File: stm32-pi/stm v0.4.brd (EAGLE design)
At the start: 128.9 x 105.8 mm, 144 parts, among them Q1 MMBT3906, Q2 MMBT3904, Q3 MMBT3904, Y1 32.768kHz

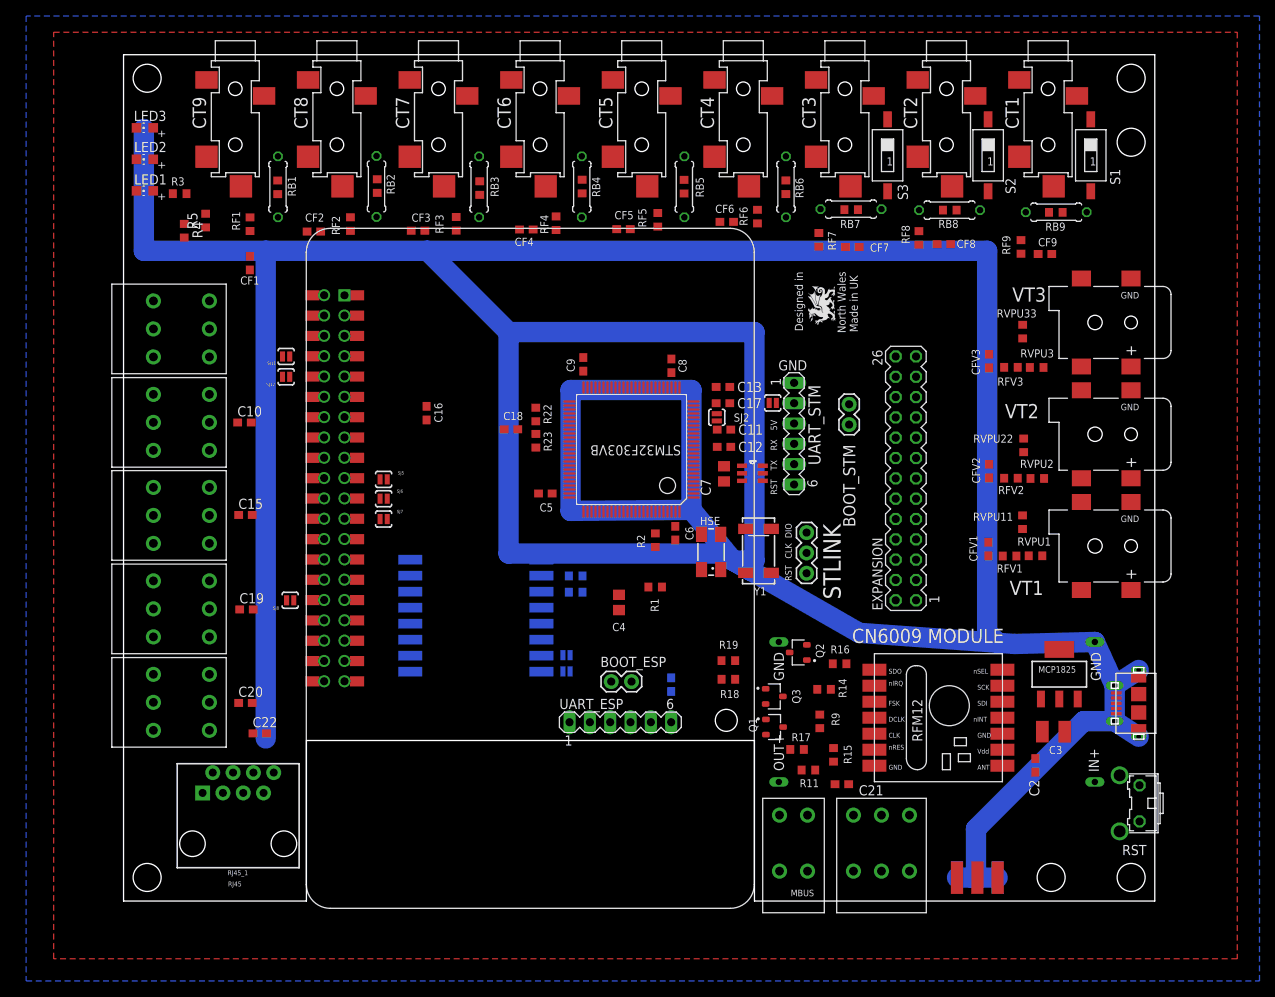
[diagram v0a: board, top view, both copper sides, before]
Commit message: update v0.4
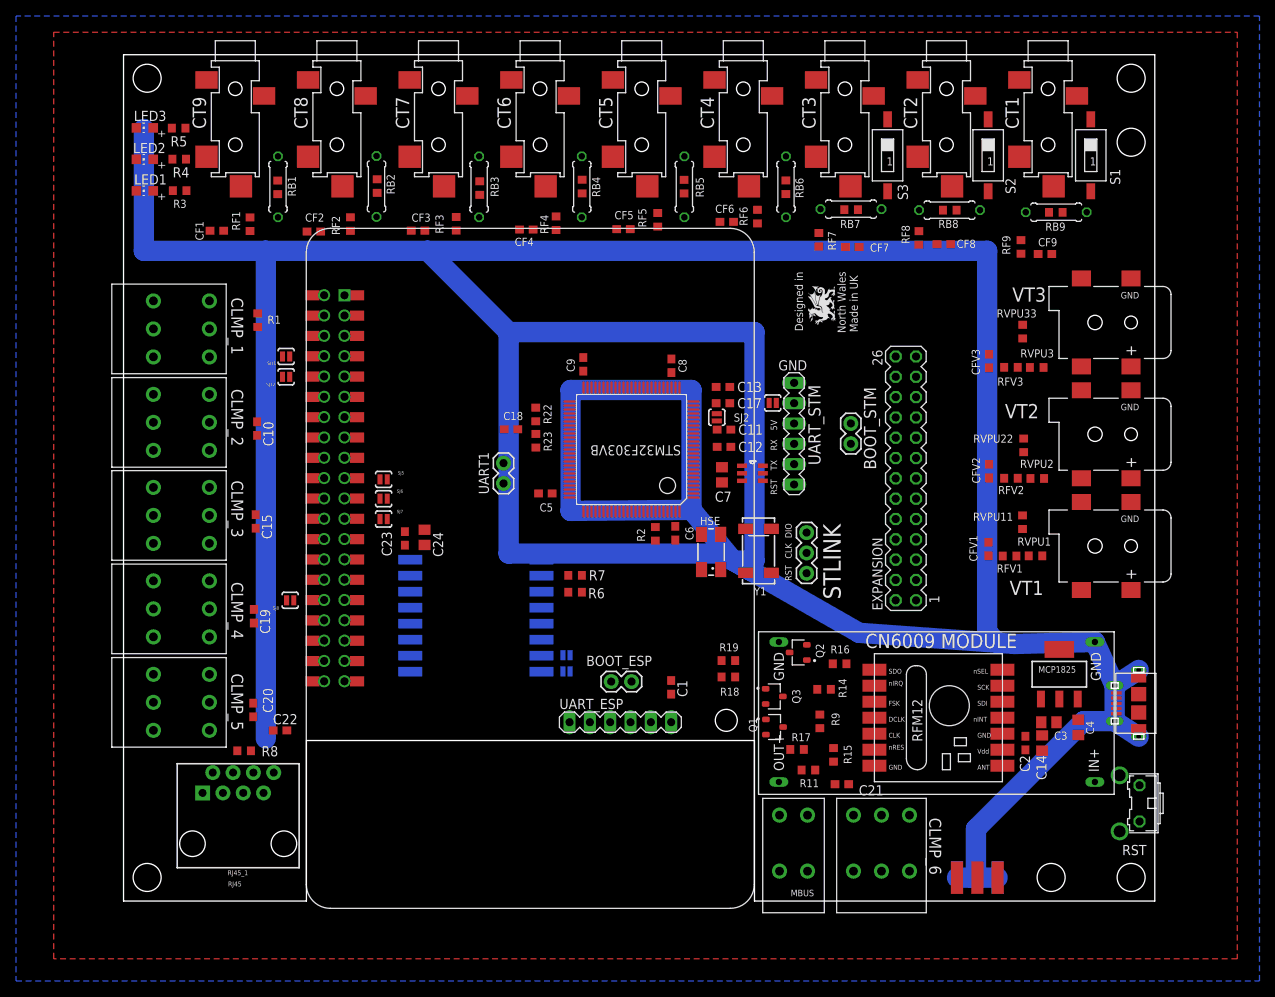
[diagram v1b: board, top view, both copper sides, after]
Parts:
- removed C16: 100nF, resistor:C0603
- added C14: 1uF, rcl:C0805
- added C23: 100nF, resistor:C0603
- added C24: 47uF, rcl:C0805
- added R8: 4.7k, resistor:R0603
- added UART1: (no value), SparkFun:1X02
- C3: device rcl:C1210 -> rcl:C0805
- UART_STM: device con-lstb:MA06-1 -> con-lstb-db:MA06-1
- moved R1 59.8 mm to (16.8, 72.6), turned to 90 degrees
- moved C4 59.5 mm to (119.3, 21.7)
- moved R5 12.0 mm to (6.89, 96.6), turned to 0 degrees
- moved R4 8.97 mm to (6.96, 92.7), turned to 0 degrees
- moved CF1 5.77 mm to (11.7, 83.8), turned to 0 degrees
- moved BOOT_STM 4.94 mm to (90.9, 57.2), turned to 90 degrees
- moved C2 3.05 mm to (112.7, 19.7), turned to 90 degrees
- moved C22 2.57 mm to (19.6, 21.3)
- moved C10 1.76 mm to (16.7, 59.1), turned to 270 degrees
- moved C15 1.52 mm to (16.5, 47.4), turned to 270 degrees
- moved C20 1.32 mm to (16.2, 23.9), turned to 270 degrees
- moved C3 1.32 mm to (115.7, 22.3)
- moved C19 1.25 mm to (16.3, 35.6), turned to 270 degrees
- moved R2 0.79 mm to (66.5, 45.9)
- moved R3 0.38 mm to (7.02, 88.8)
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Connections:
- removed net PULSE: C16.2
- new net UART1_RX: STM32F303VB.69, UART1.1
- new net UART1_TX: STM32F303VB.68, UART1.2
- net +3V3: now also C14.1, C23.1, C24.1, R8.2
- net DS18B20_1: now also 3POLE_1.P$3, 3POLE_1.P$4, STM32F303VB.63; no longer RJ45_1.4
- net DS18B20_2: now also R8.1, RJ45_1.4; no longer 3POLE_1.P$3, 3POLE_1.P$4
- net GND: now also C14.2, C23.2, C24.2; no longer C16.1
- net PULSE2: now also STM32F303VB.67
- net PUSHIN_1: now also STM32F303VB.95
- net PUSHIN_2: now also STM32F303VB.64
- net PUSHIN_3: now also STM32F303VB.65
- net PUSHIN_4: now also STM32F303VB.66
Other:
- board text added: "CLMP_1"
- board text added: "CLMP_2"
- board text added: "CLMP_3"
- board text added: "CLMP_4"
- board text added: "CLMP_5"
- board text added: "CLMP_6"

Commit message: v0.4 update
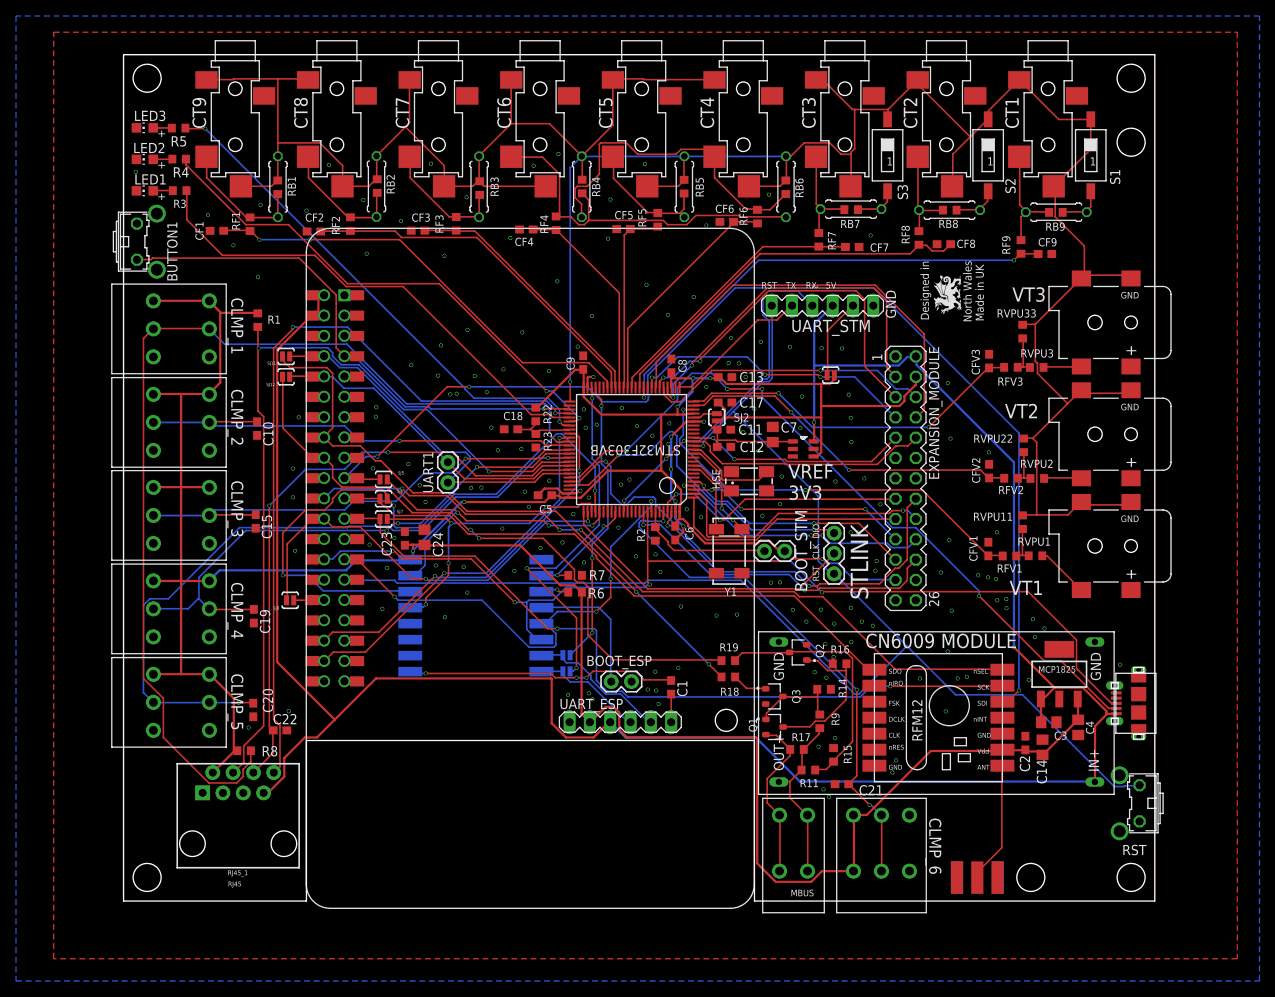
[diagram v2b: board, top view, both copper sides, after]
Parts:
- removed EXPANSION: (no value), con-lstb:MA13-2
- removed U$8: MCP1501T-33E, MCP1501T-33E:SOT95P280X145-6N
- added BUTTON1: (no value), switch-omron:B3F-31XX
- added EXPANSION_MODULE: (no value), con-lstb:MA13-2
- added VREF_3V3: MCP1501T-33E, MCP1501T-33E:SOT95P280X145-6N
- moved BOOT_STM 17.2 mm to (80.1, 43.7), turned to 0 degrees
- moved UART_STM 16.4 mm to (87.4, 74.4), turned to 180 degrees
- moved HSE 10.0 mm to (78.2, 52.5), turned to 0 degrees
- moved C7 8.11 mm to (81.2, 58.3), turned to 90 degrees
- moved SJ1 8.04 mm to (88.4, 65.7), turned to 0 degrees
- moved UART1 6.95 mm to (40.5, 52.3)
- moved Y1 3.67 mm to (75.7, 43.7)
- moved STLINK 3.44 mm to (88.8, 46.0)
- moved C13 1.25 mm to (75.2, 65.5)
- moved C14 0.53 mm to (114.9, 19.2)
- moved C17 0.28 mm to (75.2, 62.3)
- moved C5 0.23 mm to (52.7, 50.7)
- moved C9 0.22 mm to (57.5, 67.3)
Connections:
- removed net DS18B20_1: 3POLE_1.P$3, 3POLE_1.P$4, R1.1, STM32F303VB.63
- removed net N$14: EXPANSION.5
- removed net N$15: EXPANSION.7
- removed net N$17: EXPANSION.9
- removed net N$18: EXPANSION.11
- removed net N$19: EXPANSION.13
- removed net N$20: EXPANSION.15
- removed net N$21: EXPANSION.17
- removed net N$23: EXPANSION.19
- removed net N$25: EXPANSION.21
- removed net N$9: EXPANSION.1
- removed net PULSE1: C22.1, RJ45_1.6
- new net BUTTON1: BUTTON1.2, PCB2.P$47, PCB2.P$7, STM32F303VB.53
- new net DS18B20_RJ45: R1.1, RJ45_1.4, STM32F303VB.66
- new net I010_EX: EXPANSION_MODULE.24
- new net I011_EX: EXPANSION_MODULE.25
- new net IO11_EX: STM32F303VB.95
- new net IO1_EX: EXPANSION_MODULE.15, STM32F303VB.97
- new net IO2_EX: EXPANSION_MODULE.16, STM32F303VB.98
- new net IO3_EX: EXPANSION_MODULE.17, STM32F303VB.1
- new net IO4_EX: EXPANSION_MODULE.18, STM32F303VB.2
- new net IO5_EX: EXPANSION_MODULE.19, STM32F303VB.3
- new net IO6_EX: EXPANSION_MODULE.20, STM32F303VB.4
- new net IO7_EX: EXPANSION_MODULE.21, STM32F303VB.5
- new net IO8_EX: EXPANSION_MODULE.22, STM32F303VB.91
- new net PULSE1_RJ45: C22.1, RJ45_1.6, STM32F303VB.67
- new net RPI_GPIO16: PCB2.P$36, PCB2.P$76, STM32F303VB.59
- new net RPI_GPIO20: PCB2.P$38, PCB2.P$78, STM32F303VB.60
- new net SCK: ESP12.GPIO5, EXPANSION_MODULE.23, PCB2.P$28, PCB2.P$68, STM32F303VB.92
- new net SDA: ESP12.GPIO4, PCB2.P$27, PCB2.P$67, STM32F303VB.93
- new net VT1_EX: EXPANSION_MODULE.11
- new net VT2_EX: EXPANSION_MODULE.12
- new net VT3_EX: EXPANSION_MODULE.13
- net +3V3: now also EXPANSION_MODULE.4, VREF_3V3.4; no longer U$8.4
- net +3V3_ADC: now also VREF_3V3.1; no longer U$8.1
- net +5V: now also EXPANSION_MODULE.2, VREF_3V3.6; no longer U$8.6
- net CT1_EX: now also EXPANSION_MODULE.3
- net CT2_EX: now also EXPANSION_MODULE.6
- net CT3_EX: now also EXPANSION_MODULE.5
- net CT4_EX: now also EXPANSION_MODULE.8
- net CT5_EX: now also EXPANSION_MODULE.7
- net CT6_EX: now also EXPANSION_MODULE.10
- net CT7_EX: now also EXPANSION_MODULE.9
- net DS18B20_2: now also 3POLE_1.P$3, 3POLE_1.P$4, STM32F303VB.61; no longer RJ45_1.4
- net GND: now also BUTTON1.1, EXPANSION_MODULE.1, EXPANSION_MODULE.14, EXPANSION_MODULE.26, VREF_3V3.2, VREF_3V3.3, VREF_3V3.5; no longer U$8.2, U$8.3, U$8.5
- net N$13: now also PCB2.P$26, PCB2.P$66; no longer EXPANSION.3
- net NRST: now also PCB2.P$29, PCB2.P$69
- net PULSE2: now also STM32F303VB.65; no longer STM32F303VB.67
- net PUSHIN_1: now also STM32F303VB.96; no longer STM32F303VB.95
- net PUSHIN_2: now also STM32F303VB.62; no longer STM32F303VB.64
- net PUSHIN_3: now also STM32F303VB.63; no longer STM32F303VB.65
- net PUSHIN_4: now also STM32F303VB.64; no longer STM32F303VB.66
- net SPI3_CS: now also PCB2.P$24, PCB2.P$64
- net UART1_RX: now also PCB2.P$48, PCB2.P$8, SJ11.1
- net UART1_TX: now also PCB2.P$10, PCB2.P$50, SJ12.1
- net USART3_RX: no longer PCB2.P$48, PCB2.P$8, SJ11.1
- net USART3_TX: no longer PCB2.P$10, PCB2.P$50, SJ12.1
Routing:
- net GND: track 533.8 -> 29.1 mm, vias 0 -> 180
- net +3V3: track 0.00 -> 430.2 mm, vias 0 -> 5
- net BIAS: track 0.00 -> 374.6 mm, vias 0 -> 1
- net +5V: track 0.00 -> 286.9 mm, vias 0 -> 2
- net NRST: track 0.00 -> 178.4 mm, vias 0 -> 1
- net MOSI: track 0.00 -> 144.5 mm, vias 0 -> 3
- net DS18B20_2: track 0.00 -> 128.8 mm, vias 0 -> 1
- net DS18B20_RJ45: track 0.00 -> 103.8 mm, vias 0 -> 2
- net SPI_CLK: track 0.00 -> 96.8 mm, vias 0 -> 2
- net ADC_RJ45IN: track 0.00 -> 96.7 mm, vias 0 -> 2
- net CS_RFM69: track 0.00 -> 96.2 mm, vias 0 -> 3
- net SCK: track 0.00 -> 93.4 mm, vias 0 -> 4
- net D-: track 0.00 -> 93.0 mm, vias 0 -> 4
- net D+: track 0.00 -> 87.3 mm, vias 0 -> 2
- net PULSE2: track 0.00 -> 86.6 mm, vias 0 -> 2
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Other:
- board text added: "VREF 3V3"

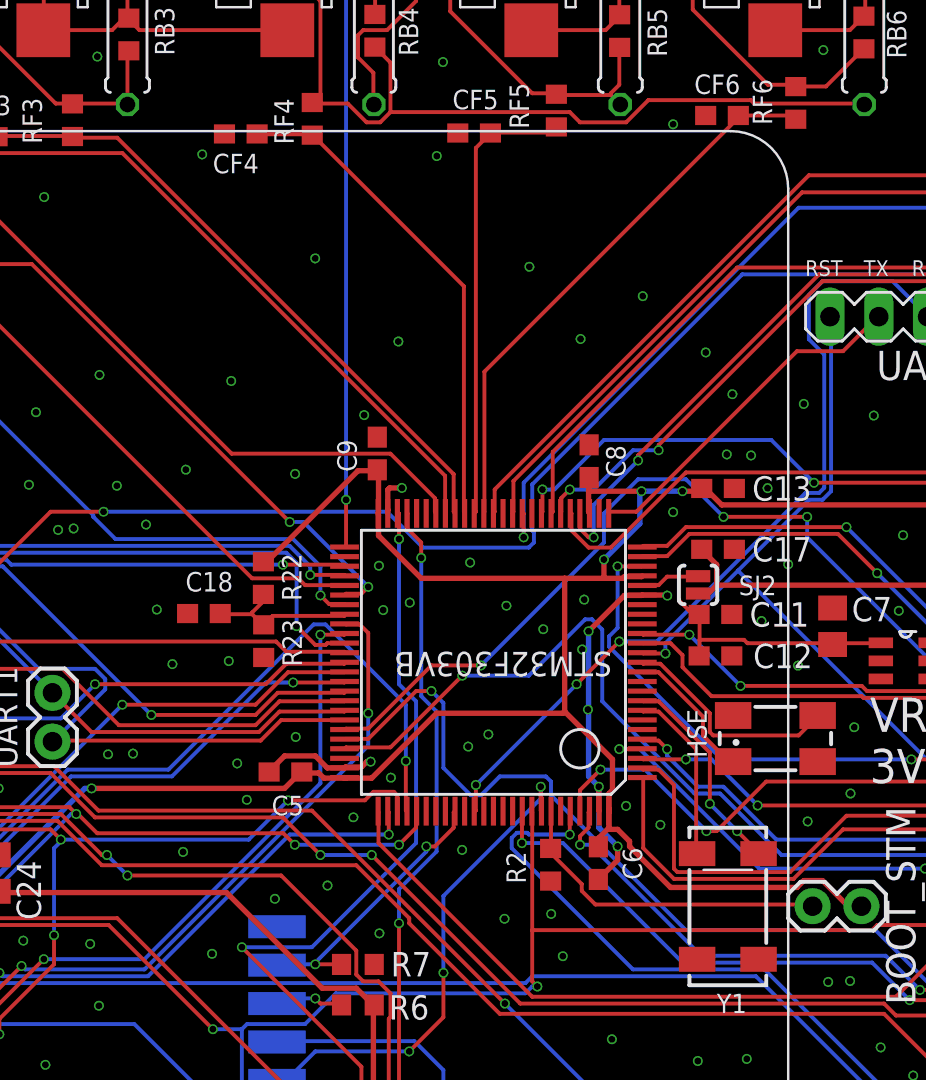
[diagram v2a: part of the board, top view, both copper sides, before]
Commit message: v0.4 update
checked
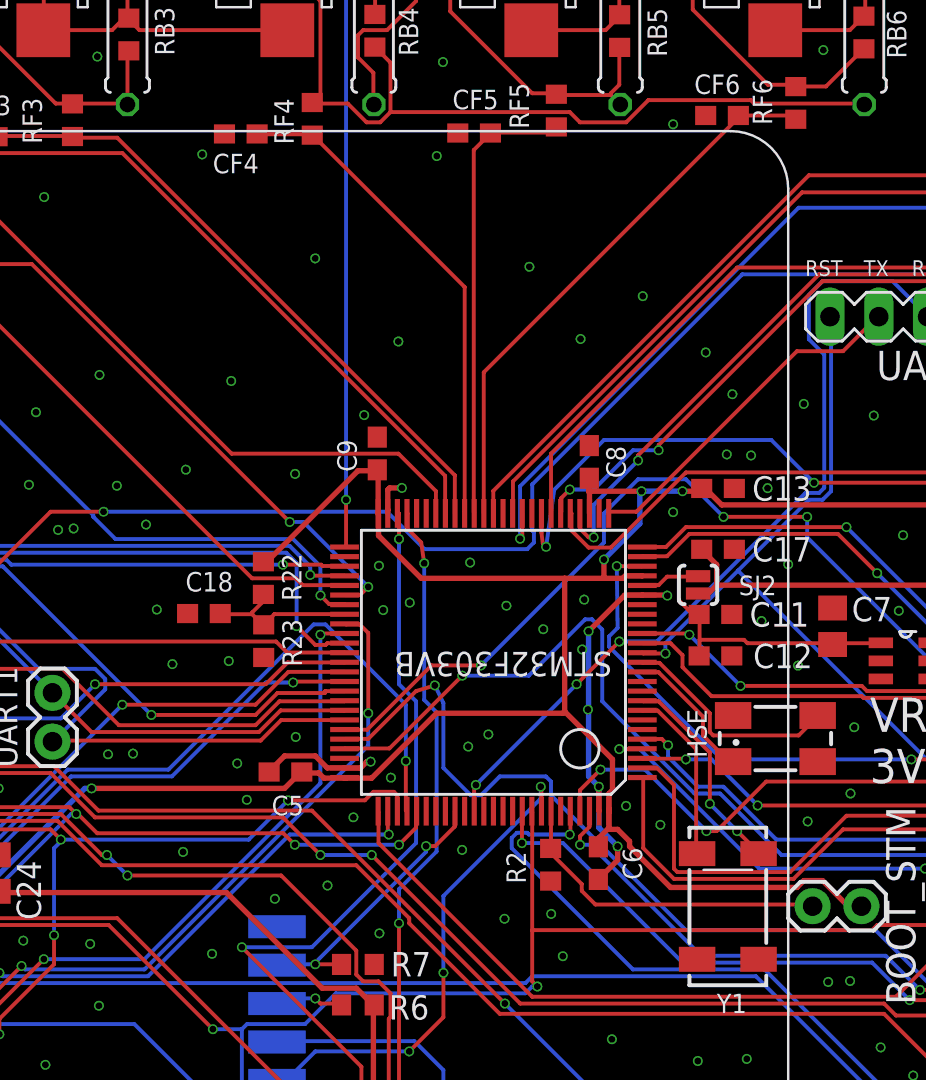
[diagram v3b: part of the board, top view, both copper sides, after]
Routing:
- net CT5_EX: track 35.9 -> 38.9 mm
